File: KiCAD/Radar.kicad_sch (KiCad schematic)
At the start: 19 parts, among them U1 LM324N_NOPB, U2 LM324N_NOPB, U3 HB100, U4 NUCLEO-L432KC

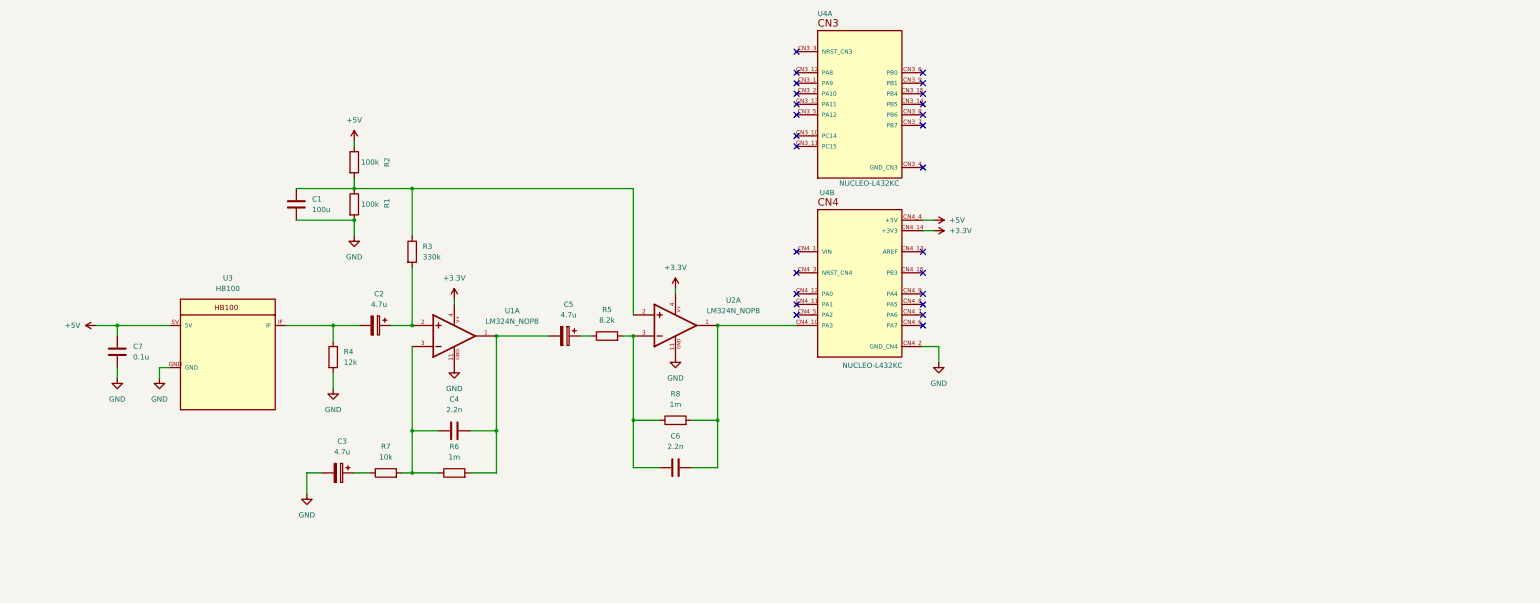
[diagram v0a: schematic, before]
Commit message: Layout V2
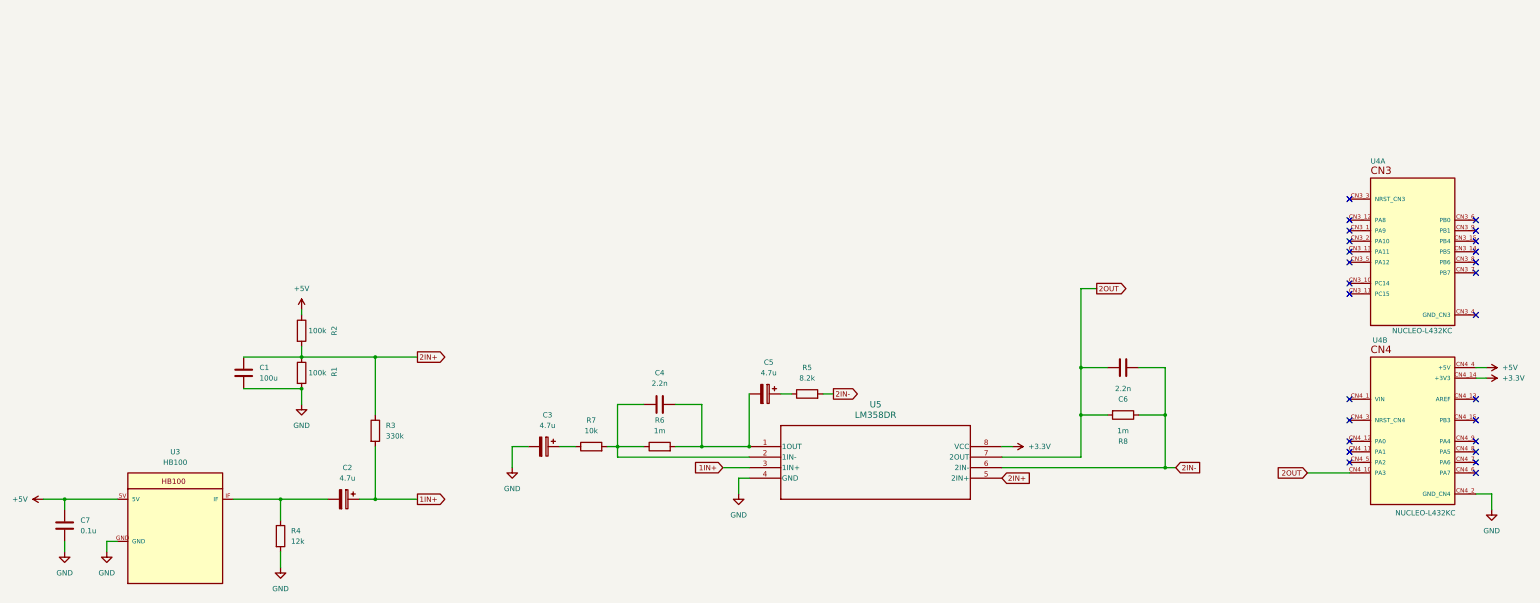
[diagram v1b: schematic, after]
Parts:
- removed U1, U2: LM324N_NOPB, LM324N_NOPB:DIP825W47P254L1917H533Q14, symbol LM324:LM324N_NOPB
- added U5: LM358DR, D8, symbol Radar:LM358DR
- U3: footprint HB100:HB100 -> Footprinty:HB100
- U4: footprint NUCLEO-L432KC:MODULE_NUCLEO-L432KC -> Footprinty:MODULE_NUCLEO-L432KC
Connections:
- net +3.3V: now also U5.8 (VCC)
- net GND: now also U5.4 (GND)
- net at C4.1, R6.1, R7.2: now also U5.2 (1IN-)
- net at C4.2, C5.2, R6.2: now also U5.1 (1OUT)
- net 2OUT: now reaches C6.2, R8.2, U4.CN4_10 (PA3)
- net 2OUT: now also U5.7 (2OUT)
- net 2IN+: now reaches C1.1, R1.1, R2.2, R3.1
- net 2IN+: now also U5.5 (2IN+)
- net 2IN-: now reaches C6.1, R5.2, R8.1
- net 2IN-: now also U5.6 (2IN-)
- net 1IN+: now reaches C2.1, R3.2
- net 1IN+: now also U5.3 (1IN+)
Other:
- moved on the sheet: C1, C2, C3, C4, C5, C6, C7, R1, R2, R3, R4, R5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
